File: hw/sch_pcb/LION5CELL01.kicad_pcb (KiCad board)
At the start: 2 copper layers, 162.1 x 85.9 mm, 207 parts, among them IC1 MAX14502AETL+, IC2 TMUX1574DYYR, J1 USBC_USB4105-GF-A, J11 SD_Card-FPS009-4200-0, J2 46436-9327, J6 HEADER_2x03, Q1 BC817-25, Q2 BC817-25, Q3 BC817-25, Q5 BC817-25, Q6 BC817-25, U10 SN74HC164D, U11 TPS22965-Q1, U12 ATMEGA1284P-AU, U13 AT24CS64-SSHM, U14 PCF85263A, U15 TPS631000DRLR, U16 TPS631000DRLR, U17 TPS631000DRLR, U2 USBLC6-2SC6, U3 FT260Q-T, U4 SHT35-DIS, U5 PCA9541ABS/01, U7 TCA4307, U8 BQ34Z100, U9 BQ25628E, Y1 8 MHz, Y2 ABS07-120-32.768KHZ-T

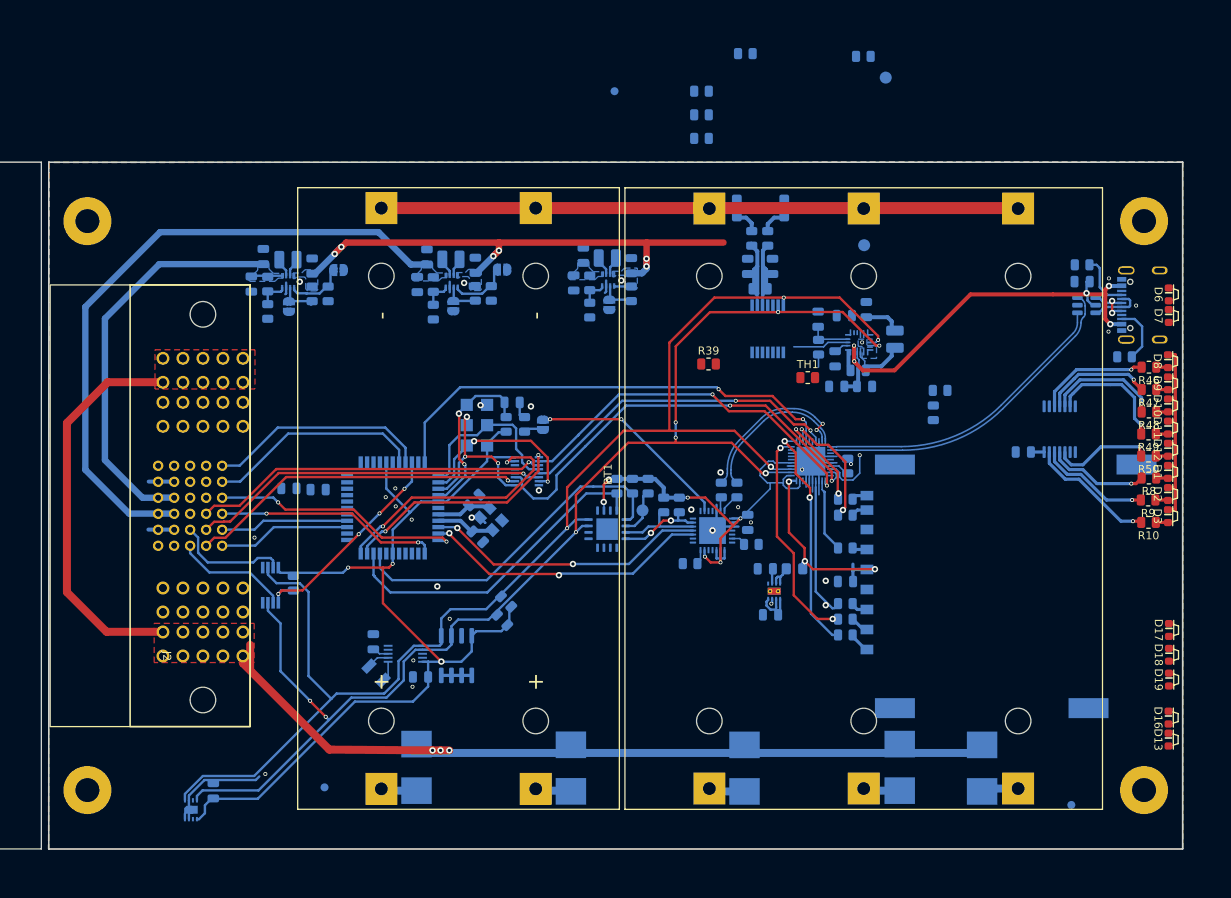
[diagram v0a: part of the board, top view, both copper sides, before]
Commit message: wip, layout improvements
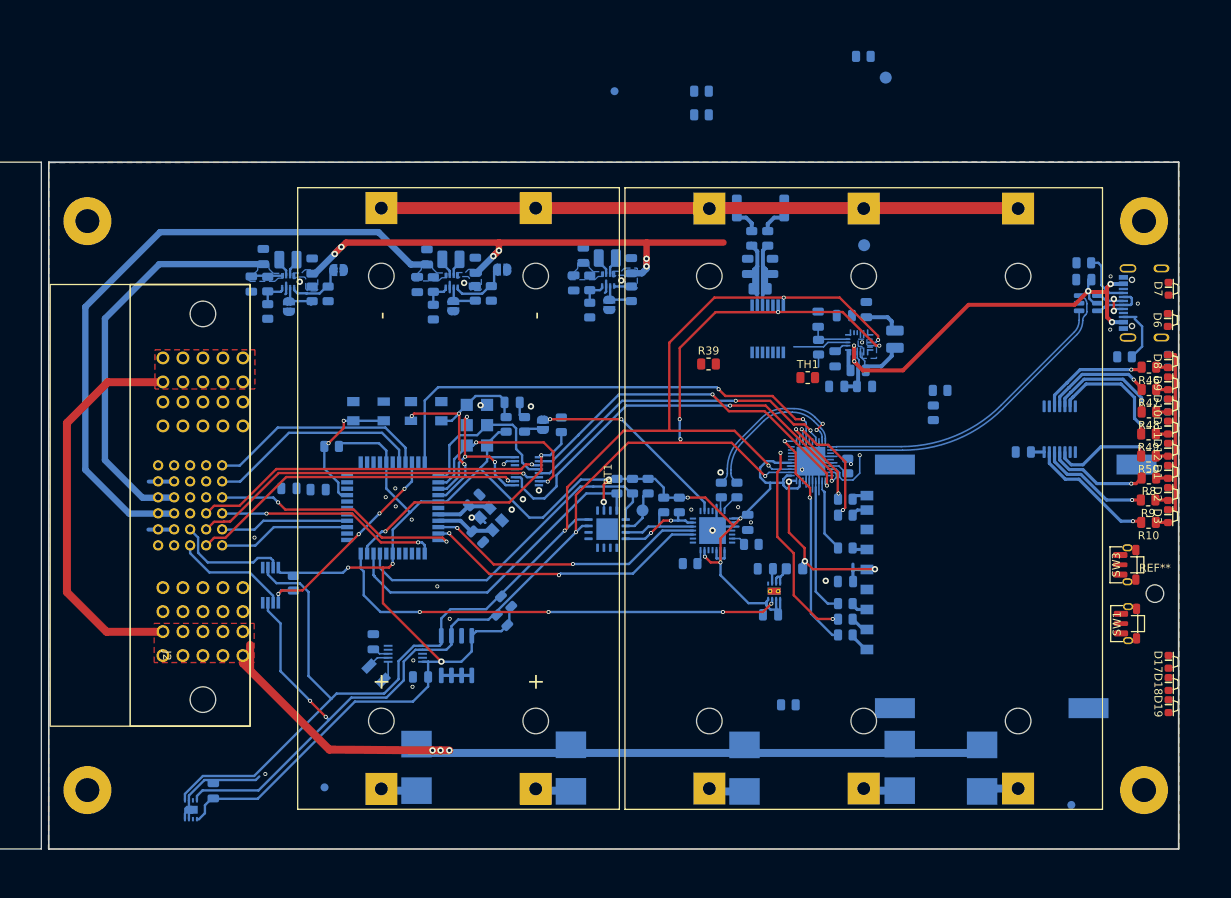
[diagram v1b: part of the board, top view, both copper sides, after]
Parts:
- added R11: 10k, Resistor_SMD:R_0805_2012Metric, B.Cu at (141.7, 94.9)
- added REF**: MountingHole_2.2mm_M2, MountingHole:MountingHole_2.2mm_M2, F.Cu at (215.9, 116.0)
- added SW1: SW_Push, Mlab_SW:SKRT, F.Cu at (211.7, 119.8)
- added SW2: MCU_RST, Mlab_SW:KMT031 NGJ LHS C&K, B.Cu at (124.8, 93.2)
- added SW3: SW_Push, Mlab_SW:SKRT, F.Cu at (211.6, 112.4)
- added SW4: SW_Push, Mlab_SW:KMT031 NGJ LHS C&K, B.Cu at (117.6, 93.2)
- D1, D12, D2, D3: value ORAGE -> GREEN
- D13, D16: moved to B.Cu
- D8, D9: value ORAGE -> RED
- moved R40 81.6 mm to (170.1, 129.9)
- moved R78 60.2 mm to (113.0, 97.6)
- moved D13 47.4 mm to (217.5, 86.9), turned to 90 degrees
- moved D16 39.0 mm to (217.5, 92.5), turned to 90 degrees
- moved D17 3.98 mm to (217.6, 124.5)
- moved D18 3.65 mm to (217.6, 127.3)
- moved D7 3.40 mm to (217.6, 77.9)
- moved D19 3.33 mm to (217.6, 130.1)
- moved D6 3.20 mm to (217.5, 81.8)
- moved J1 0.33 mm to (216.7, 79.7)
- moved U2 0.33 mm to (207.6, 79.7)
- moved C1 0.33 mm to (207.0, 76.8)
- moved R1 0.33 mm to (207.0, 74.7)
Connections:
- net /mcu/CCLK1 renamed /mcu/CCLK
- net /mcu/CCMD1 renamed /mcu/CCMD
- net /mcu/CDAT1_0 renamed /mcu/CDAT0
- net /mcu/CDAT1_1 renamed /mcu/CDAT1
- net /mcu/CDAT1_2 renamed /mcu/CDAT2
- net /mcu/CDAT1_3 renamed /mcu/CDAT3
- net /mcu/SCK_MCU renamed /mcu/SCLK_MCU
- net /mcu/SCK_SD renamed /mcu/SCLK_SD
- net EXT_SCK renamed EXT_SCLK
- IC2 pad 15: /mcu/SPI_MUX_EN -> GND
- U12 pad 22: /mcu/SPI_MUX_EN -> 3v3_SD_CTRL
- U12 pad 43: 3v3_SD_CTRL -> unconnected-(U12-(PCINT11/AIN1/OC0)PB3-Pad43)
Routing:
- net 3v3_SD_CTRL: track 0.65 -> 58.3 mm, vias 1 -> 4
- net +3.3V: track 185.8 -> 223.8 mm
- net /mcu/SPI_MUX_EN: track 32.5 -> 0.00 mm, vias 2 -> 0
- net /mcu/BTN_USER_B: track 0.00 -> 17.2 mm, vias 0 -> 2
- net /mcu/RST#_P: track 21.6 -> 30.8 mm, vias 2 -> 3
- net /mcu/SPI_MUX_SEL: track 28.5 -> 33.5 mm
- net /mcu/CDAT3: track 27.6 -> 25.6 mm
- net /mcu/CS_SD: track 58.7 -> 60.3 mm
- net GND: track 60.6 -> 62.1 mm, vias 30 -> 32
- net /mcu/MISO_MCU: track 21.9 -> 23.2 mm
- net /liion/A: track 14.0 -> 13.3 mm
- net /liion/B: track 13.8 -> 13.3 mm
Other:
- board size 162.1 x 85.9 mm -> 161.6 x 85.9 mm
